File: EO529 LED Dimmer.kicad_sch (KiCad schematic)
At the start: 59 parts, among them J1 VBat, Q1 BC639, Q2 BC639, Q3 BC639, Q4 BC639, U1 NE556, U2 NE556, U3 LM393, U4 LM393

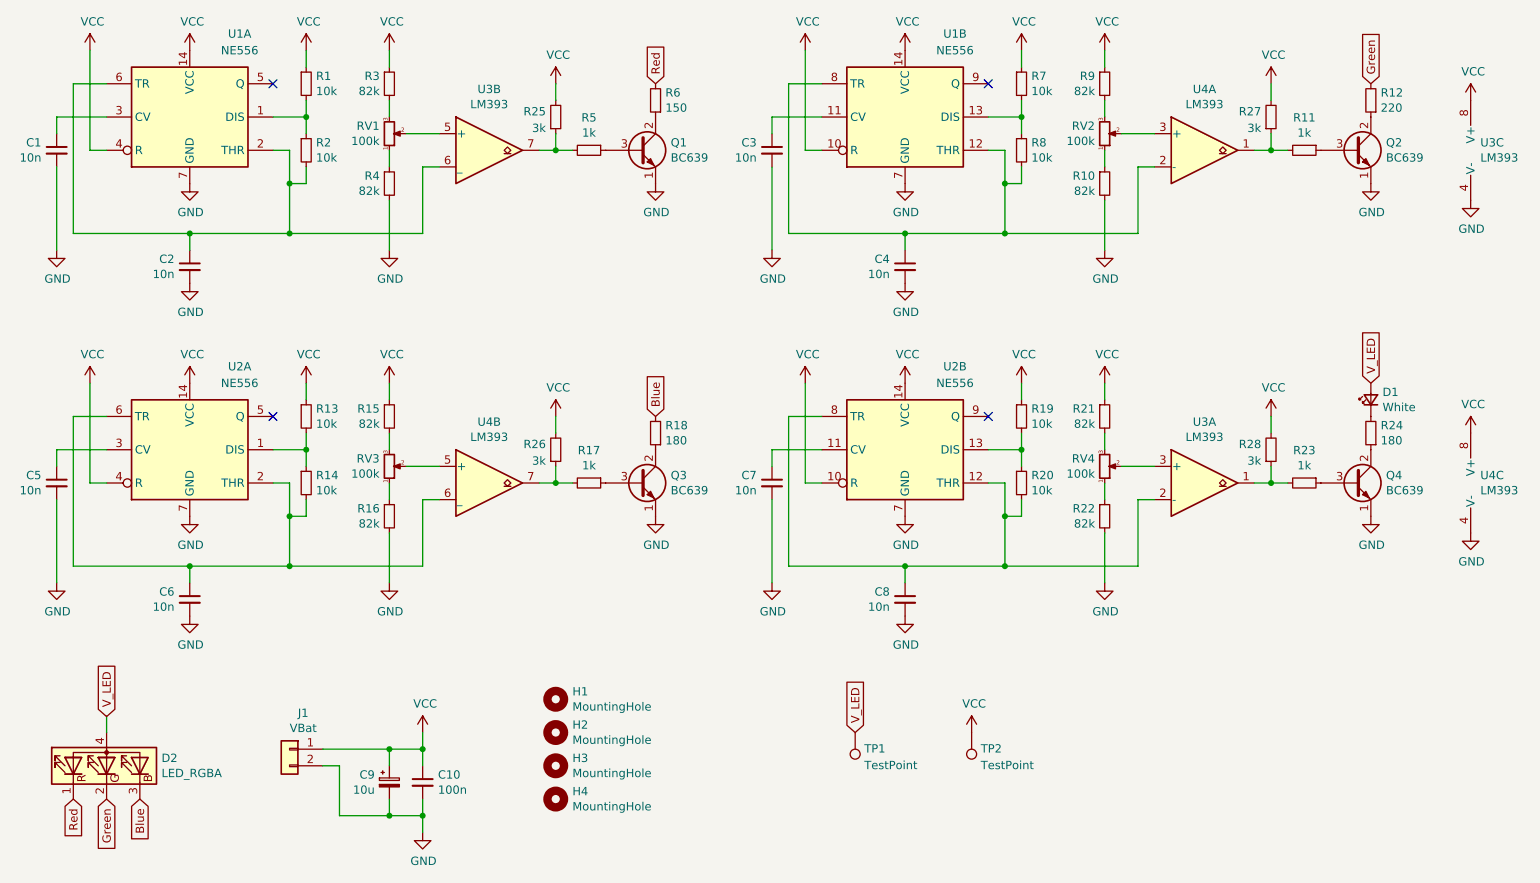
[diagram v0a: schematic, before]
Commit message: Final revision
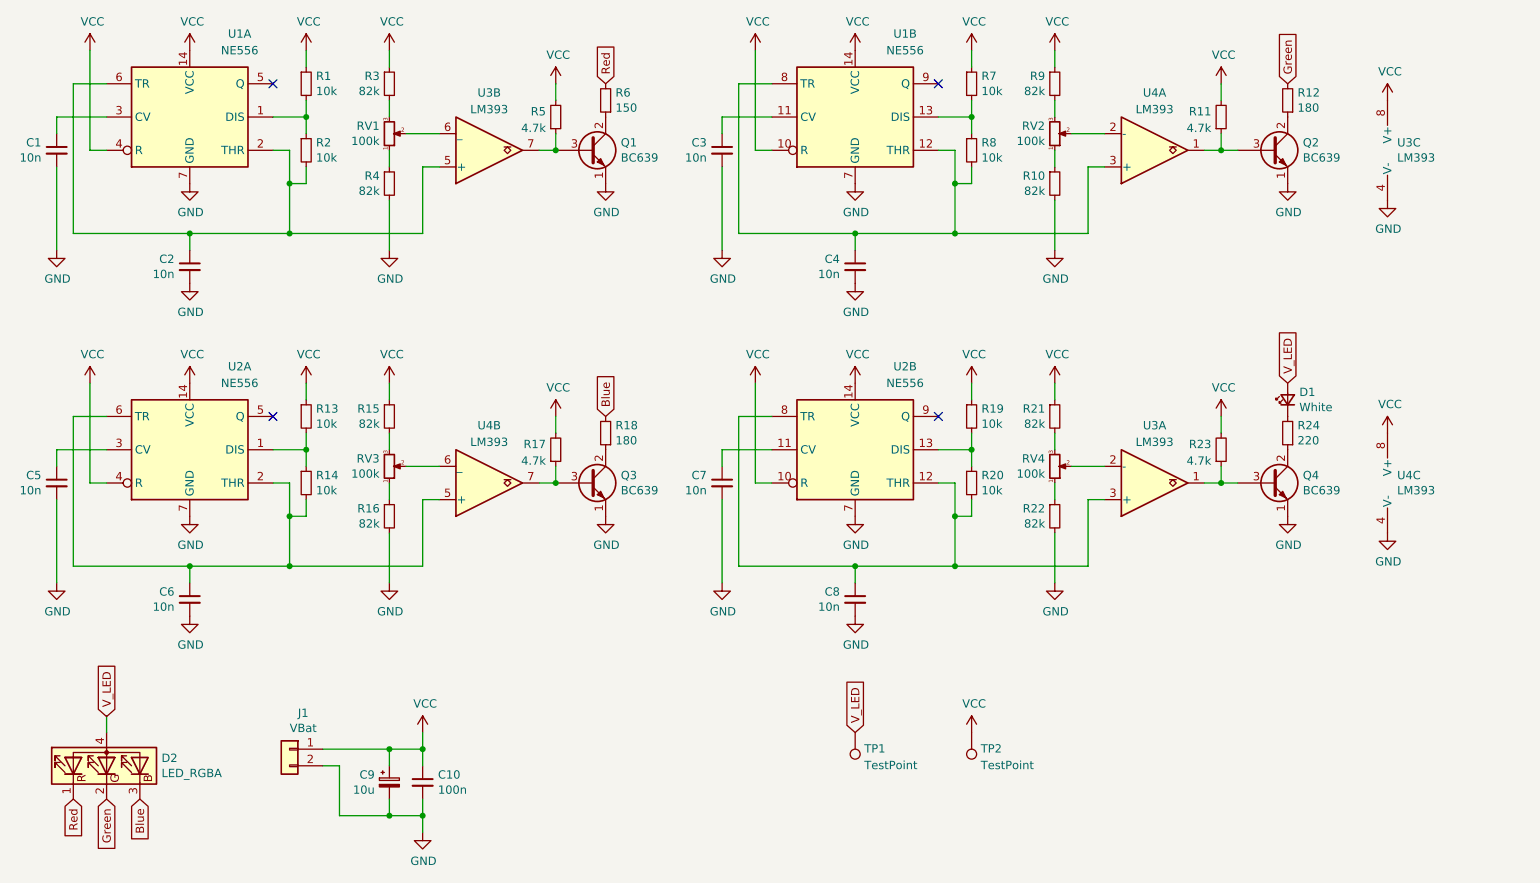
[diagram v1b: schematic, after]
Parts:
- removed H1, H2, H3, H4: MountingHole, MountingHole:MountingHole_2.2mm_M2, symbol Mechanical:MountingHole
- removed R11, R17, R23, R5: 1k, Resistor_THT:R_Axial_DIN0207_L6.3mm_D2.5mm_P7.62mm_Horizontal, symbol Device:R_Small
- R11: renamed from R27; value 3k -> 4.7k
- R12: value 220 -> 180; footprint Resistor_THT:R_Axial_DIN0207_L6.3mm_D2.5mm_P7.62mm_Horizontal -> Resistor_THT:R_Axial_DIN0414_L11.9mm_D4.5mm_P15.24mm_Horizontal
- R17: renamed from R26; value 3k -> 4.7k
- R18, R6: footprint Resistor_THT:R_Axial_DIN0207_L6.3mm_D2.5mm_P7.62mm_Horizontal -> Resistor_THT:R_Axial_DIN0414_L11.9mm_D4.5mm_P15.24mm_Horizontal
- R23: renamed from R28; value 3k -> 4.7k
- R24: value 180 -> 220; footprint Resistor_THT:R_Axial_DIN0207_L6.3mm_D2.5mm_P7.62mm_Horizontal -> Resistor_THT:R_Axial_DIN0414_L11.9mm_D4.5mm_P15.24mm_Horizontal
- R5: renamed from R25; value 3k -> 4.7k
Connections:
- net at C2.1, R2.2, U1.2 (THR)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: now also U3.5 (+); no longer U3.6 (_)
- net at RV1.2: now also U3.6 (_); no longer U3.5 (+)
- net at Q1.3 (B): now also R5.1, U3.7
- net at C4.1, R8.2, U1.12 (THR)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: now also U4.3 (+); no longer U4.2 (-)
- net at Q2.3 (B): now also R11.1, U4.1
- net at RV2.2: now also U4.2 (-); no longer U4.3 (+)
- net at U4.5 (+): now also C6.1, R14.2, U2.2 (THR), U2.6 (TR); no longer RV3.2
- net at R17.1, U4.7: now also Q3.3 (B)
- net at C8.1, R20.2, U2.12 (THR)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: now also U3.3 (+); no longer U3.2 (-)
- net at Q4.3 (B): now also R23.1, U3.1
- net at RV4.2: now also U3.2 (-); no longer U3.3 (+)
- new net: RV3.2, U4.6 (_)
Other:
- moved on the sheet: C3, C4, C7, C8, D1, Q1, Q2, Q3, Q4, R10, R11, R12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

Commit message: Revert "Final revision"
This reverts commit 9e4e9cd728e1364b963bc449a0773ff88f127e0e.
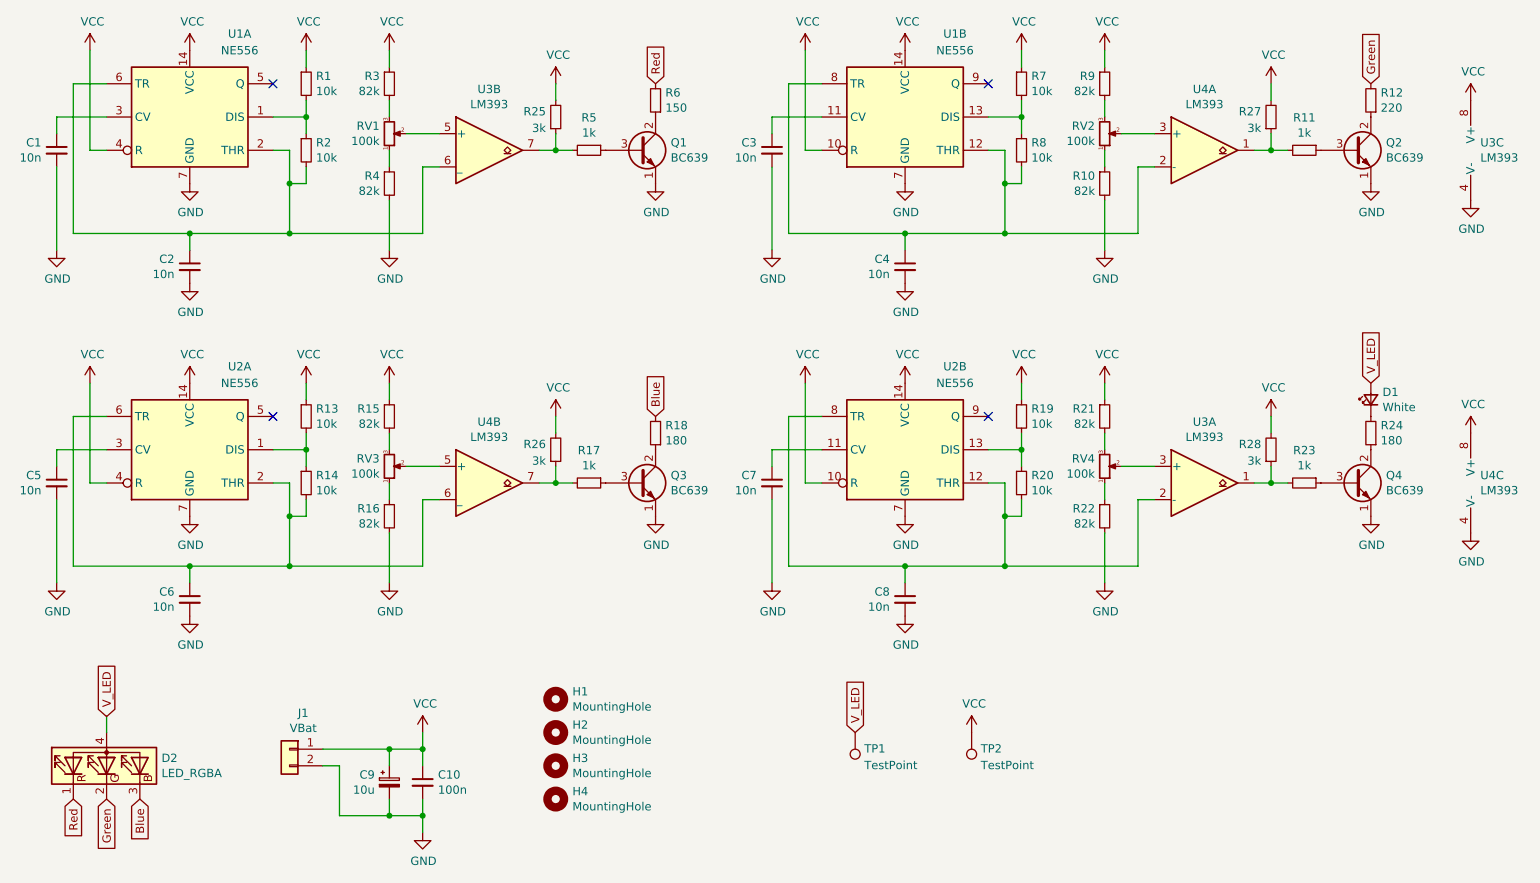
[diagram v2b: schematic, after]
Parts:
- added H1, H2, H3, H4: MountingHole, MountingHole:MountingHole_2.2mm_M2, symbol Mechanical:MountingHole
- added R11, R17, R23, R5: 1k, Resistor_THT:R_Axial_DIN0207_L6.3mm_D2.5mm_P7.62mm_Horizontal, symbol Device:R_Small
- R12: value 180 -> 220; footprint Resistor_THT:R_Axial_DIN0414_L11.9mm_D4.5mm_P15.24mm_Horizontal -> Resistor_THT:R_Axial_DIN0207_L6.3mm_D2.5mm_P7.62mm_Horizontal
- R18, R6: footprint Resistor_THT:R_Axial_DIN0414_L11.9mm_D4.5mm_P15.24mm_Horizontal -> Resistor_THT:R_Axial_DIN0207_L6.3mm_D2.5mm_P7.62mm_Horizontal
- R24: value 220 -> 180; footprint Resistor_THT:R_Axial_DIN0414_L11.9mm_D4.5mm_P15.24mm_Horizontal -> Resistor_THT:R_Axial_DIN0207_L6.3mm_D2.5mm_P7.62mm_Horizontal
- R25: renamed from R5; value 4.7k -> 3k
- R26: renamed from R17; value 4.7k -> 3k
- R27: renamed from R11; value 4.7k -> 3k
- R28: renamed from R23; value 4.7k -> 3k
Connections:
- net at C2.1, R2.2, U1.2 (THR)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: now also U3.6 (_); no longer U3.5 (+)
- net at RV1.2: now also U3.5 (+); no longer U3.6 (_)
- net at R25.1, U3.7: now also R5.2; no longer Q1.3 (B)
- net at C4.1, R8.2, U1.12 (THR)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: now also U4.2 (-); no longer U4.3 (+)
- net at RV2.2: now also U4.3 (+); no longer U4.2 (-)
- net at R27.1, U4.1: now also R11.2; no longer Q2.3 (B)
- net at C6.1, R14.2, U2.2 (THR)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: now also U4.6 (_); no longer U4.5 (+)
- net at RV3.2: now also U4.5 (+); no longer U4.6 (_)
- net at R26.1, U4.7: now also R17.2; no longer Q3.3 (B)
- net at C8.1, R20.2, U2.12 (THR)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: now also U3.2 (-); no longer U3.3 (+)
- net at RV4.2: now also U3.3 (+); no longer U3.2 (-)
- net at R28.1, U3.1: now also R23.2; no longer Q4.3 (B)
- new net: Q1.3 (B), R5.1
- new net: Q2.3 (B), R11.1
- new net: Q3.3 (B), R17.1
- new net: Q4.3 (B), R23.1
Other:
- moved on the sheet: C3, C4, C7, C8, D1, Q1, Q2, Q3, Q4, R10, R12, R18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
